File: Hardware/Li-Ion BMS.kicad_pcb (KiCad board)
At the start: 2 copper layers, 34 x 34 mm, 54 parts, among them IC1 MAX17320, J10 Battery, J11 Conn_01x02, J2 Conn_01x04_Male, J3 Conn_01x02_Male, J4 Conn_01x02_Male, J5 Conn_01x02_Male, J6 Conn_01x02_Male, J7 Conn_01x08_Male, J9 QWIIC_Stack_II, Q1 AO3401A, Q2 AO3400, Q3 SiSF06DN

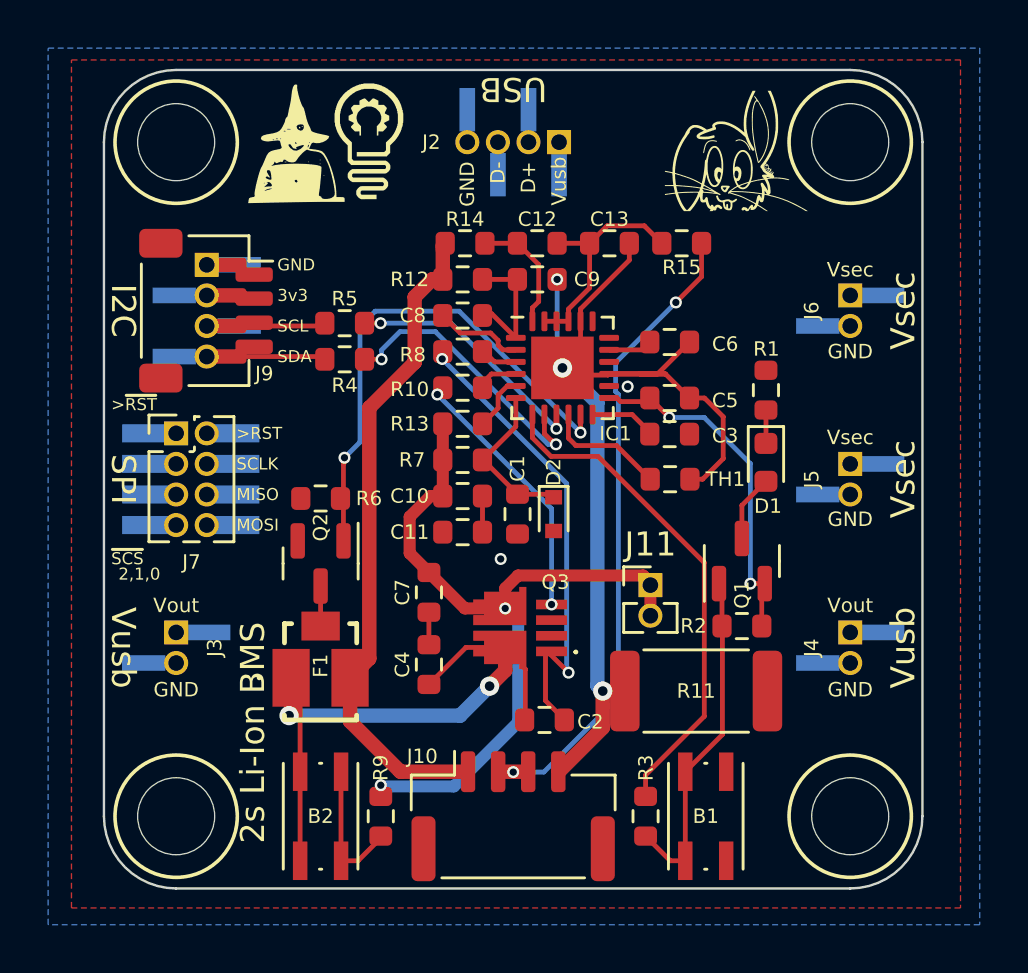
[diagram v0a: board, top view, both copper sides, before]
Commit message: ...
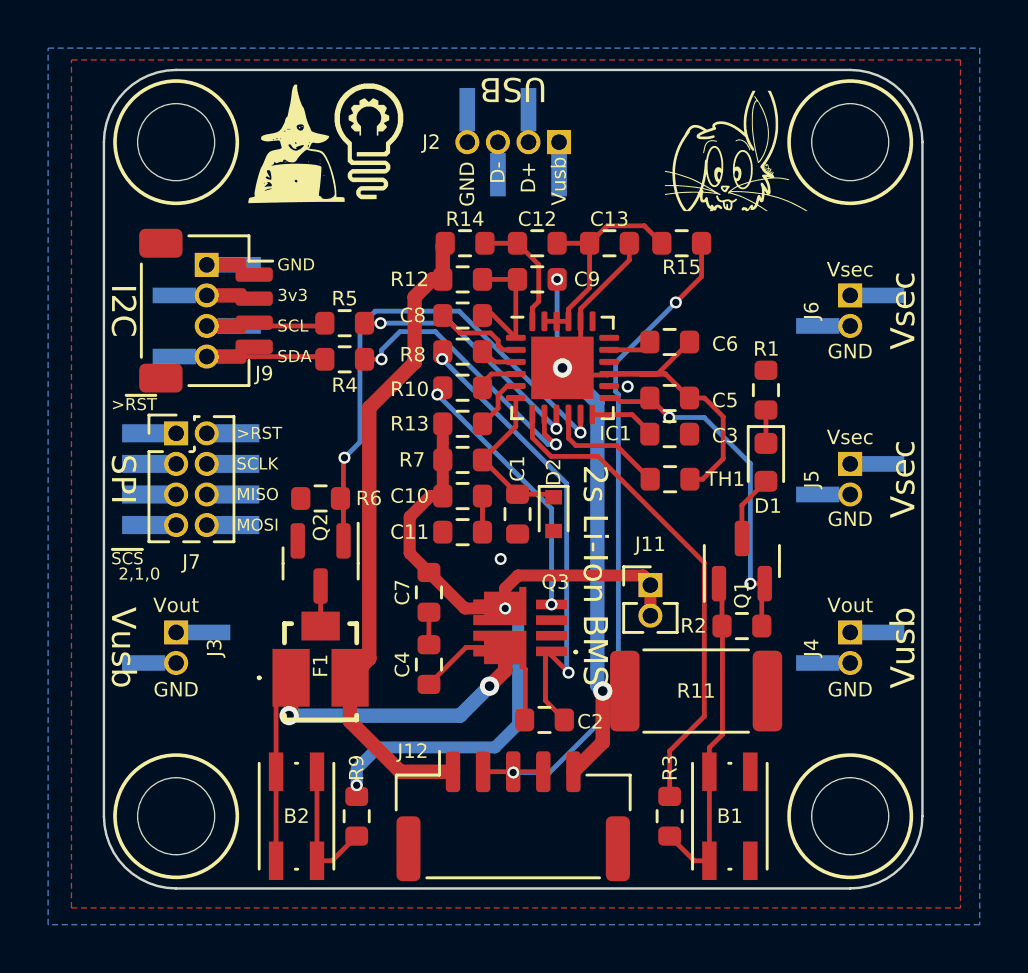
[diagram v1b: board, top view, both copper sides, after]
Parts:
- removed J10: Battery, Connector_JST:JST_GH_SM04B-GHS-TB_1x04-1MP_P1.25mm_Horizontal
- added J12: Conn_01x05_MountingPin, Connector_JST:JST_GH_SM05B-GHS-TB_1x05-1MP_P1.25mm_Horizontal, F.Cu at (100.0, 114.0)
- moved B1 1.00 mm to (109.0, 114.0)
- moved B2 1.00 mm to (91.0, 114.0)
- moved R3 1.00 mm to (106.5, 114.0)
- moved R9 1.00 mm to (93.5, 114.0)
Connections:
- net /batts renamed batts
- net /cell1 renamed cell3
- R15 pad 2: /cell -> cell
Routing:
- net cell: track 0.00 -> 28.7 mm, vias 0 -> 2
- net /cell: track 27.3 -> 0.00 mm, vias 2 -> 0
- net VBUS: track 31.4 -> 32.8 mm
- net +BATT: track 27.5 -> 26.9 mm
